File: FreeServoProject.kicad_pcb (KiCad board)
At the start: 2 copper layers, 54 parts, among them J1 4P-SBN, J2 Conn_01x03, J3 Conn_01x04, J4 Conn_01x04, M1 Motor_DC, U1 AP7381-33Y-13, U2 STM32F303K8Tx, U3 VNH7070BASTR, U4 74LVC1G125, U5 74LVC1G126, U6 ST1480ACDR, U7 AS5600-ASOM

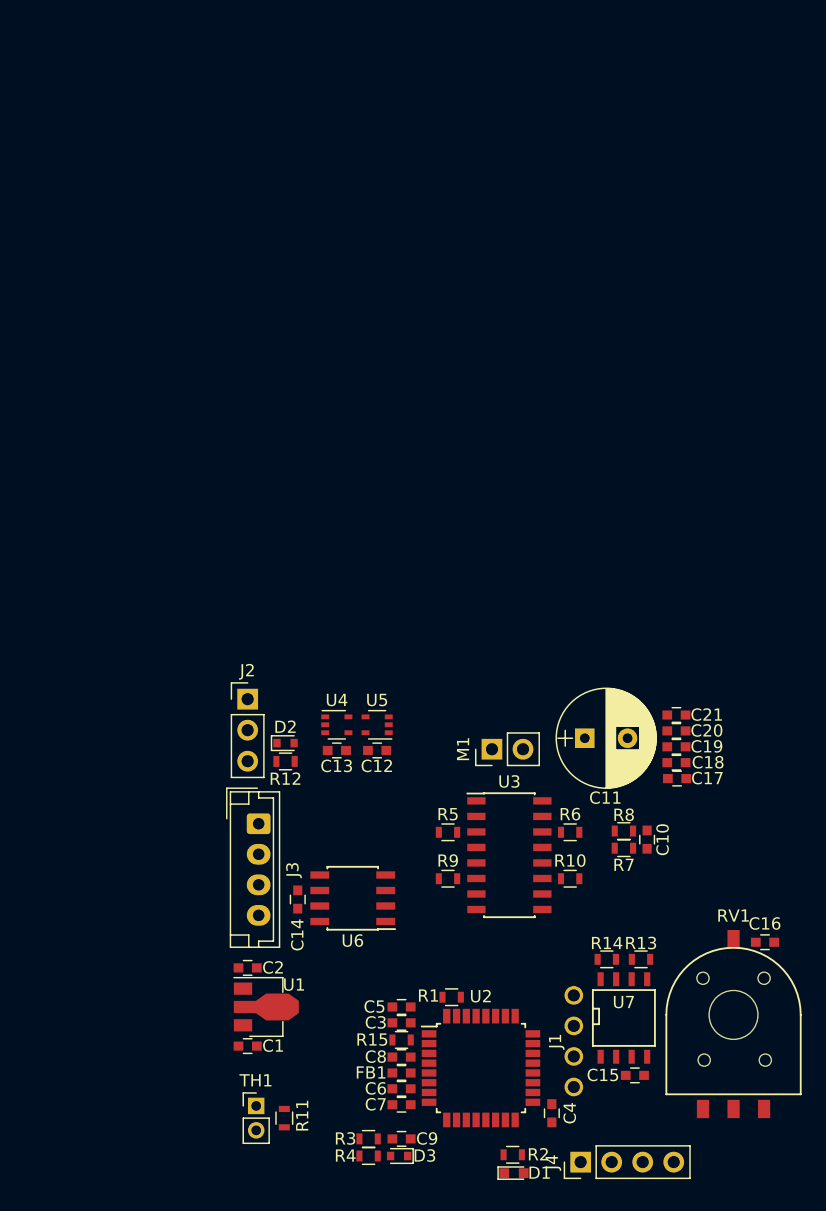
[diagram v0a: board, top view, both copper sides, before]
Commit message: Add files via upload
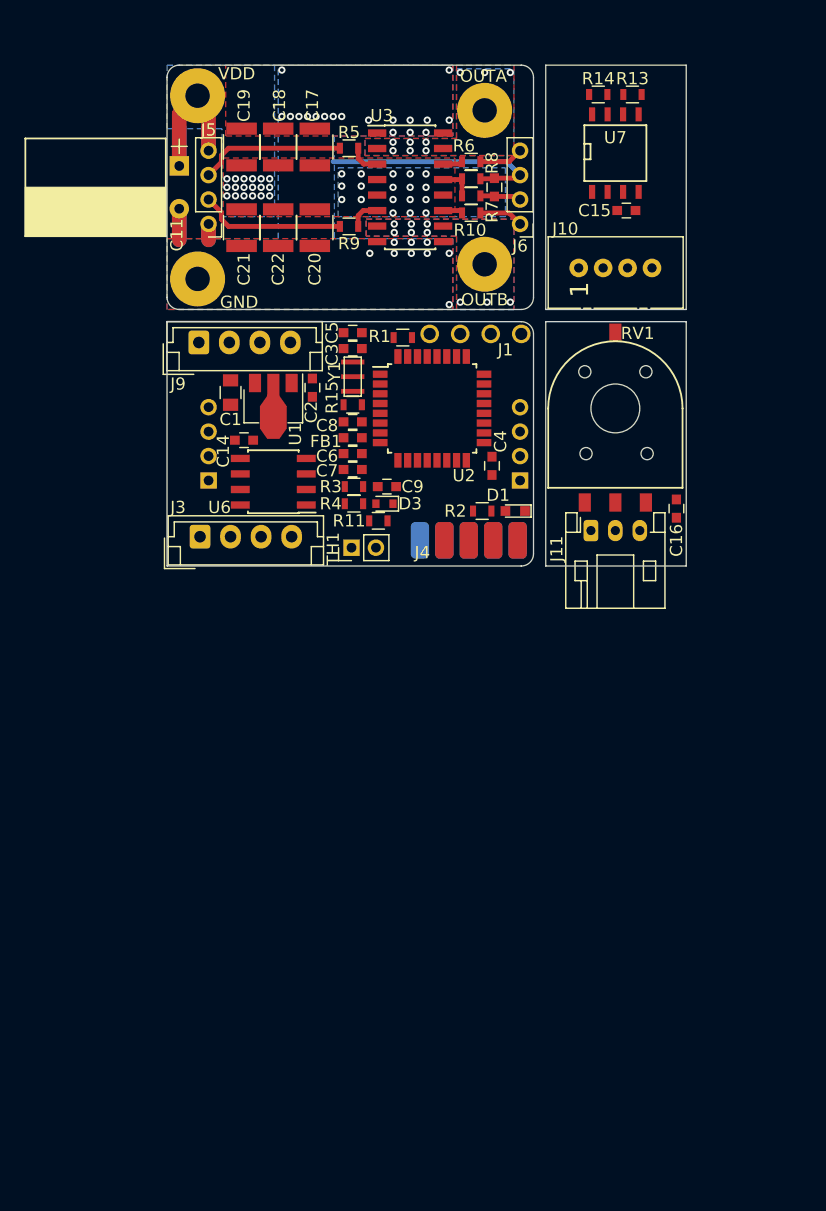
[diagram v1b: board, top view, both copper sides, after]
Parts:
- removed C12, C13: 0.1u, Capacitors_SMD:C_0603
- removed D2: D_TVS, Diodes_SMD:D_SOD-523
- removed J2: Conn_01x03, Pin_Headers:Pin_Header_Straight_1x03_Pitch2.54mm
- removed M1: Motor_DC, Pin_Headers:Pin_Header_Straight_1x02_Pitch2.54mm
- removed R12: 10k, Resistors_SMD:R_0603
- removed U4: 74LVC1G125, TO_SOT_Packages_SMD:SOT-353_SC-70-5
- removed U5: 74LVC1G126, TO_SOT_Packages_SMD:SOT-353_SC-70-5
- added C22: 10u35V, Capacitors_SMD:C_1210, F.Cu at (124.1, 72.3)
- added H1: MountingHole_Pad, Wire_Pads:SolderWirePad_single_2mmDrill, F.Cu at (141.0, 62.7)
- added H2: MountingHole_Pad, Wire_Pads:SolderWirePad_single_2mmDrill, F.Cu at (141.0, 75.3)
- added H3: MountingHole_Pad, Wire_Pads:SolderWirePad_single_2mmDrill, F.Cu at (117.5, 61.5)
- added H4: MountingHole_Pad, Wire_Pads:SolderWirePad_single_2mmDrill, F.Cu at (117.5, 76.5)
- added J10: Conn_01x04, Connect:Grove_1x04, F.Cu at (148.7, 75.6)
- added J11: S3B-PH-K, Connectors_JST:JST_PH_S3B-PH-K_1x03_P2.00mm_Horizontal, F.Cu at (149.7, 97.1)
- added J12: 5_SMD_Pad, SMD_Pad:5_SMD_Pad, B.Cu at (139.7, 97.9)
- added J5: Pin_Header_Straight_1x04_Pitch2.00mm, Pin_Headers:Pin_Header_Straight_1x04_Pitch2.00mm, F.Cu at (118.4, 72.0)
- added J6: Pin_Header_Straight_1x04_Pitch2.00mm, Pin_Headers:Pin_Header_Straight_1x04_Pitch2.00mm, F.Cu at (143.9, 72.0)
- added J7: Socket_Strip_Straight_1x04_Pitch2.00mm, Socket_Strips:Socket_Strip_Straight_1x04_Pitch2.00mm, B.Cu at (118.4, 93.0)
- added J8: Socket_Strip_Straight_1x04_Pitch2.00mm, Socket_Strips:Socket_Strip_Straight_1x04_Pitch2.00mm, B.Cu at (143.9, 93.0)
- added J9: Conn_01x04, Connectors_JST:JST_EH_B4B-EH-A_1x04_P2.50mm_Vertical, F.Cu at (117.6, 81.7)
- added Y1: Resonator, CSTNE8M00G55Z000R0:CSTNE8M00G55Z000R0, F.Cu at (127.9, 84.5)
- C1: footprint Capacitors_SMD:C_0603 -> Capacitors_SMD:C_0805
- C11: footprint Capacitors_ThroughHole:CP_Radial_D8.0mm_P3.50mm -> 35ZLH220MEFC8X11.5:CP_Radial_D8.0mm_P3.50mm
- C17, C18, C19, C20, C21: footprint Capacitors_SMD:C_0603 -> Capacitors_SMD:C_1210
- J4: value Conn_01x04 -> 4_SMD_Pad; footprint Pin_Headers:Pin_Header_Straight_1x04_Pitch2.54mm -> SMD_Pad:4_SMD_Pad
- R8: value 1.5k -> 1.5k 1%
- moved U7 70.8 mm to (151.7, 66.2)
- moved C15 70.8 mm to (152.6, 70.9)
- moved R13 70.8 mm to (153.1, 61.4)
- moved R14 70.8 mm to (150.3, 61.4)
- moved C19 60.6 mm to (121.1, 65.7), turned to 90 degrees
- moved C18 60.0 mm to (124.1, 65.7), turned to 90 degrees
- moved C17 59.6 mm to (127.1, 65.7), turned to 90 degrees
- moved J1 58.5 mm to (140.2, 81.0), turned to 180 degrees
- moved R5 56.6 mm to (129.9, 65.8)
- moved C11 56.0 mm to (116.0, 69.0), turned to 270 degrees
- moved R6 55.5 mm to (139.9, 66.9)
- moved C3 55.3 mm to (130.2, 82.2)
- moved C5 55.3 mm to (130.2, 80.9)
- moved U3 55.3 mm to (134.9, 69.0)
- moved R10 55.1 mm to (139.9, 71.1)
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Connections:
- R1 pad 1: +3V3 -> Net-(R1-Pad1)
- U2 pad 31: +3V3 -> Net-(R1-Pad1)
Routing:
- net GND: track 0.00 -> 28.2 mm, vias 0 -> 27
- net +BATT: track 0.00 -> 17.0 mm, vias 0 -> 36
- net INB: track 0.00 -> 12.4 mm
- net INA: track 0.00 -> 12.0 mm
- net CS: track 0.00 -> 4.08 mm
- net SEL0: track 0.00 -> 3.62 mm
- net PWM: track 0.00 -> 3.62 mm
- net Net-(R7-Pad1): track 0.00 -> 2.98 mm
- net Net-(R9-Pad2): track 0.00 -> 2.61 mm
- net Net-(R5-Pad2): track 0.00 -> 2.58 mm
- net Net-(R6-Pad1): track 0.00 -> 1.63 mm
- net Net-(R10-Pad1): track 0.00 -> 1.63 mm
- net OUTB: vias 0 -> 9
- net OUTA: vias 0 -> 9
- added copper zone on B.Cu, net +BATT
- added copper zone on F.Cu, net +BATT
- added copper zone on B.Cu, net GND
- added copper zone on F.Cu, net GND
- added copper zone on B.Cu, net OUTA
- added copper zone on F.Cu, net OUTA
- added copper zone on B.Cu, net OUTB
- added copper zone on F.Cu, net OUTB
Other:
- board outline added: 42.5 x 41 mm
- net class Default: trace_width 0.25 -> 0.2; via_dia 0.8 -> 0.6; via_drill 0.4 -> 0.3
- rule trace_min: 0.2 -> 0.1524
- rule via_min_drill: 0.3 -> 0.2
- board text added: "GND"
- board text added: "OUTA"
- board text added: "OUTB"
- board text added: "VDD"

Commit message: Add files via upload
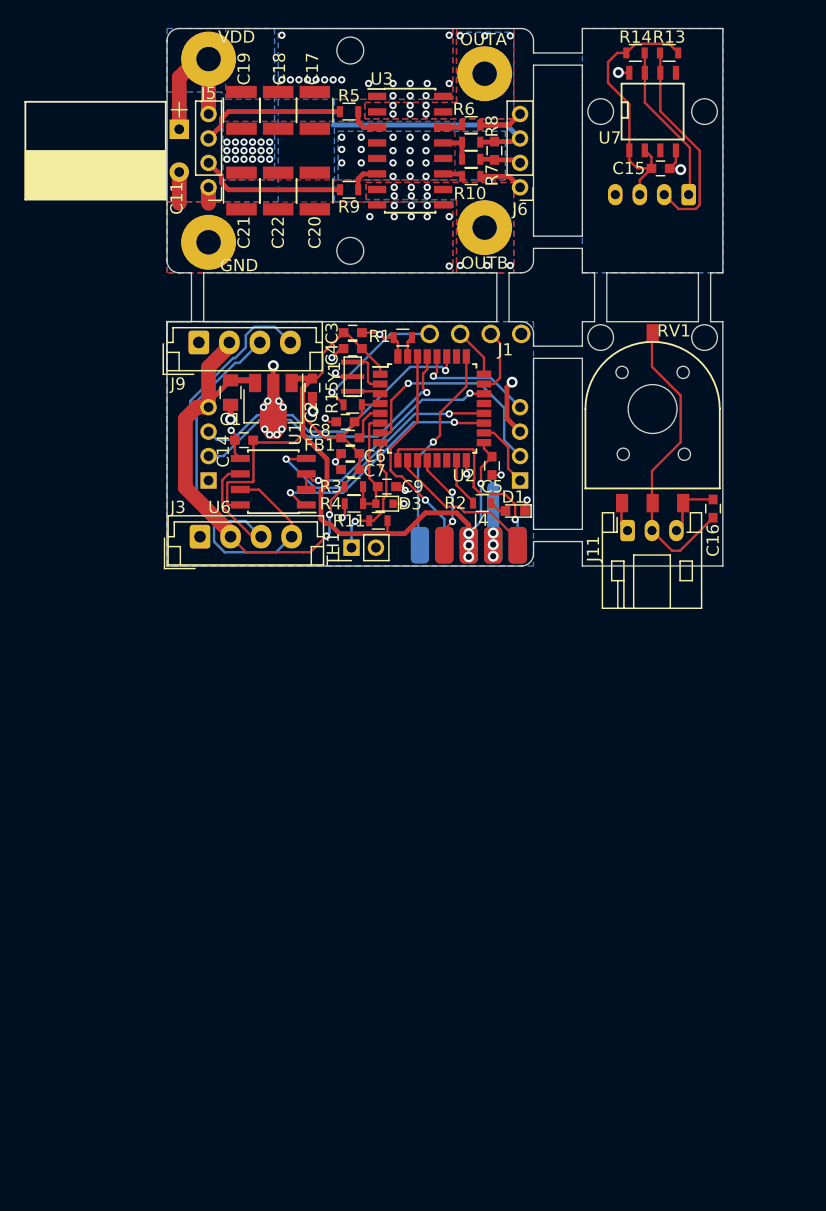
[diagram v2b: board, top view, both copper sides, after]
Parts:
- J10: value Conn_01x04 -> S4B-PH-K; footprint Connect:Grove_1x04 -> Connectors_JST:JST_PH_S4B-PH-K_1x04_P2.00mm_Horizontal; moved to B.Cu
- moved C5 15.8 mm to (141.6, 91.8), turned to 270 degrees
- moved C4 14.9 mm to (130.2, 82.2), turned to 180 degrees
- moved J10 10.8 mm to (157.7, 69.6), turned to 180 degrees
- moved U7 4.57 mm to (154.8, 62.8)
- moved R14 4.57 mm to (153.3, 58.0)
- moved R13 4.53 mm to (156.1, 58.0)
- moved C15 4.44 mm to (155.4, 67.5)
- moved H3 3.13 mm to (118.4, 58.5)
- moved H4 3.13 mm to (118.4, 73.5)
- moved RV1 3.05 mm to (154.8, 87.2)
- moved R6 3.00 mm to (139.9, 63.9)
- moved C10 3.00 mm to (141.8, 66.0)
- moved C11 3.00 mm to (116.0, 66.0)
- moved C16 3.00 mm to (159.7, 95.3)
- moved C17 3.00 mm to (127.1, 62.7)
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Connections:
- J4 pad 1: GND -> ENC_A
- J4 pad 3: ENC_A -> GND
- U2 pad 10: Net-(U2-Pad10) -> ENC_B
- U2 pad 11: ENC_A -> Net-(U2-Pad11)
- U2 pad 12: Net-(U2-Pad12) -> ENC_A
- U2 pad 26: ENC_B -> Net-(U2-Pad26)
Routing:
- net +3V3: track 0.00 -> 103.0 mm, vias 0 -> 4
- net Potentiometer: track 0.00 -> 43.0 mm, vias 0 -> 1
- net GND: track 28.2 -> 70.6 mm, vias 27 -> 56
- net +BATT: track 17.0 -> 55.1 mm, vias 36 -> 38
- net RS485_D-: track 0.00 -> 37.9 mm
- net SDA: track 0.00 -> 35.8 mm, vias 0 -> 1
- net SCL: track 0.00 -> 30.8 mm, vias 0 -> 1
- net RS485_D+: track 0.00 -> 29.4 mm
- net INA: track 12.0 -> 36.6 mm, vias 0 -> 1
- net INB: track 12.4 -> 36.8 mm, vias 0 -> 1
- net TX: track 0.00 -> 21.4 mm, vias 0 -> 2
- net RX: track 0.00 -> 20.0 mm, vias 0 -> 2
- net DE: track 0.00 -> 19.0 mm, vias 0 -> 2
- net CS: track 4.08 -> 22.7 mm, vias 0 -> 1
- net ENC_B: track 0.00 -> 12.5 mm
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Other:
- board size 42.5 x 41 mm -> 45.5 x 44 mm
- board text added: "FreeServo Project v.0.1 by Nori"
- board text added: "FreeServoProject v.0.1 by Nori"
